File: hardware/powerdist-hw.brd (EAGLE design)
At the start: 84.8 x 18 mm, 41 parts, among them IC1 AVRXDA32TQFP, IC3 ACS712, Q5 NFET SO8

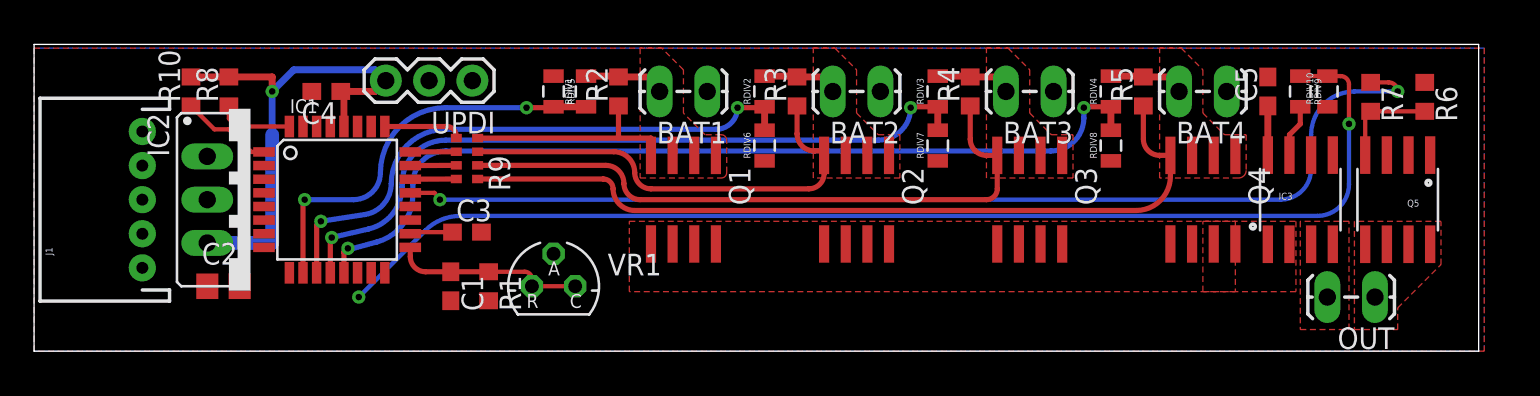
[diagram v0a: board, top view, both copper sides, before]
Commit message: layout complete
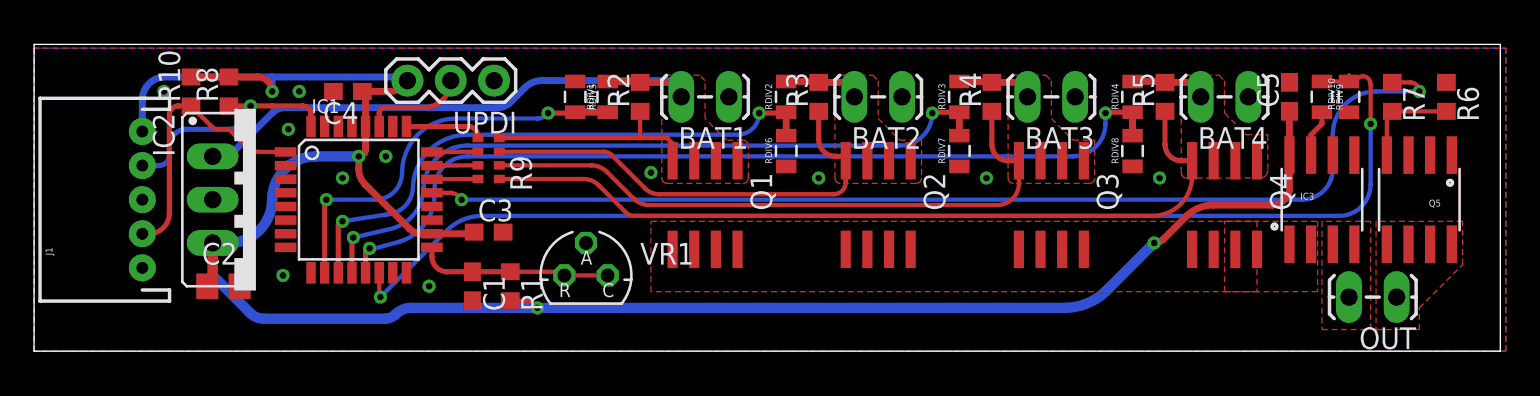
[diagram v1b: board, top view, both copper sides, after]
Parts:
- moved VR1 2.01 mm to (32.4, 4.45)
- moved BAT4 1.31 mm to (71.1, 14.9)
- moved RDIV10 1.31 mm to (77.2, 14.9)
- moved BAT1 1.31 mm to (40.6, 14.9)
- moved BAT3 1.31 mm to (61.0, 14.9)
- moved Q2 1.31 mm to (49.5, 8.57)
- moved R2 1.31 mm to (35.6, 14.9)
- moved R3 1.31 mm to (46.0, 14.9)
- moved RDIV1 1.31 mm to (33.7, 14.9)
- moved RDIV2 1.31 mm to (44.1, 14.9)
- moved RDIV4 1.31 mm to (64.5, 14.9)
- moved RDIV6 1.31 mm to (44.1, 11.7)
- moved RDIV8 1.31 mm to (64.5, 11.7)
- moved RDIV5 1.31 mm to (31.8, 14.9)
- moved BAT2 1.31 mm to (50.8, 14.9)
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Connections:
- net SCL: now also J1.2
- net SDA: now also J1.4
- net VCC: now also J1.5
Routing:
- net VCC: track 36.2 -> 128.8 mm, vias 1 -> 4
- net BAT1+: track 6.12 -> 36.2 mm
- net SCL: track 5.40 -> 15.9 mm
- net SDA: track 4.48 -> 14.0 mm, vias 0 -> 1
- net N$2: track 0.00 -> 5.77 mm
- net VLOAD: track 69.6 -> 71.5 mm
- net GATE2: track 26.6 -> 27.8 mm
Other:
- board size 84.8 x 18 mm -> 86 x 18 mm
